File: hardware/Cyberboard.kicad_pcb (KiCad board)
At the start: 4 copper layers, 51 x 21 mm, 68 parts, among them J1 Conn_01x20, J2 Conn_01x20, SW1 SW_Push, SW2 SW_Push, U1 SZYY0402Y_C434450, U10 XL-1005UBC_C22355736, U2 TPD2EUSB30, U3 NX2012SA-32.768KHZ-STD-MUB-2, U4 STM32WB55RGVx, U5 BQ24072RGT, U6 TPS631000DRLR, U7 ICM-42688-PC, U8 BMP580, U9 DFE252012P-1R0M=P2, X1 NX2016SA-32MHZ-STD-CZS-5

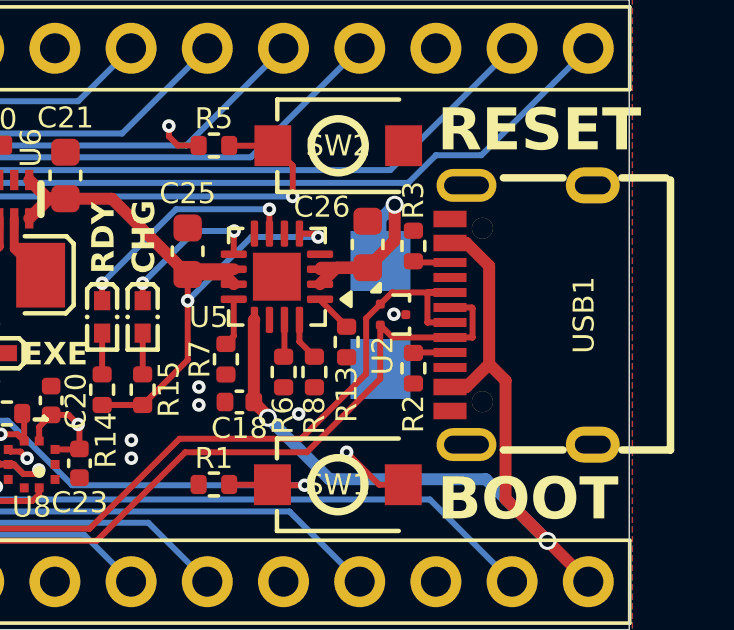
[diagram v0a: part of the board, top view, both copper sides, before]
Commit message: rounded corners and new renders and flyer
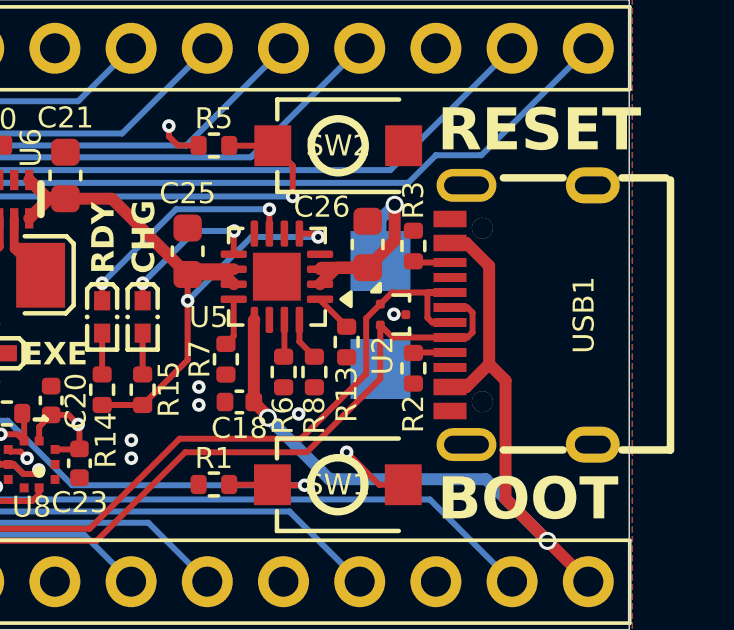
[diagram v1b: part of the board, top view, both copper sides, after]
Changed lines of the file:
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@@
+	)
+	(segment
+		(start 165.77 77.25)
+		(end 165.02 77.25)
+		(width 0.2)
+		(layer "F.Cu")
+		(net 27)
 	)
 	(segment
@@
 	)
 	(segment
+		(start 165.019 77.251)
+		(end 165.019 78.094)
+		(width 0.2)
+		(layer "F.Cu")
+		(net 27)
+	)
+	(segment
+		(start 165.019 78.094)
+		(end 165.175 78.25)
+		(width 0.2)
+		(layer "F.Cu")
+		(net 27)
+	)
+	(segment
 		(start 156.756802 82.125)
 		(end 160.806802 82.125)
@@
 	)
 	(segment
-		(start 165.77 77.25)
-		(end 165.02 77.25)
-		(width 0.2)
-		(layer "F.Cu")
-		(net 27)
-	)
-	(segment
-		(start 165.019 78.249)
-		(end 165.02 78.25)
+		(start 165.175 78.25)
+		(end 165.77 78.25)
 		(width 0.2)
 		(layer "F.Cu")
@@
 	)
 	(segment
-		(start 165.02 78.25)
-		(end 165.77 78.25)
-		(width 0.2)
-		(layer "F.Cu")
-		(net 27)
-	)
-	(segment
-		(start 165.019 77.251)
-		(end 165.019 78.249)
-		(width 0.2)
-		(layer "F.Cu")
-		(net 27)
-	)
-	(segment
 		(start 150.375 84.95)
 		(end 150.55 85.125)
@@
 	)
 	(segment
-		(start 166.521 78.749)
-		(end 166.52 78.75)
-		(width 0.2)
-		(layer "F.Cu")
-		(net 28)
-	)
-	(segment
-		(start 165.77 77.75)
-		(end 166.5 77.75)
+		(start 166.521 77.921)
+		(end 166.521 78.579)
+		(width 0.2)
+		(layer "F.Cu")
+		(net 28)
+	)
+	(segment
+		(start 166.35 77.75)
+		(end 166.521 77.921)
 		(width 0.2)
 		(layer "F.Cu")
@@
 	)
 	(segment
+		(start 165.77 77.75)
+		(end 166.35 77.75)
+		(width 0.2)
+		(layer "F.Cu")
+		(net 28)
+	)
+	(segment
 		(start 165.77 78.75)
 		(end 163.86 78.75)
@@
 	)
 	(segment
+		(start 166.35 78.75)
+		(end 165.77 78.75)
+		(width 0.2)
+		(layer "F.Cu")
+		(net 28)
+	)
+	(segment
 		(start 160.993198 82.575)
 		(end 156.943198 82.575)
@@
 	)
 	(segment
-		(start 166.521 77.771)
-		(end 166.521 78.749)
-		(width 0.2)
-		(layer "F.Cu")
-		(net 28)
-	)
-	(segment
 		(start 140.599517 85.525)
 		(end 138.036136 82.961619)
@@
 	)
 	(segment
-		(start 166.52 78.75)
-		(end 165.77 78.75)
-		(width 0.2)
-		(layer "F.Cu")
-		(net 28)
-	)
-	(segment
-		(start 166.5 77.75)
-		(end 166.521 77.771)
-		(width 0.2)
-		(layer "F.Cu")
-		(net 28)
-	)
-	(segment
 		(start 163.4475 78.3375)
 		(end 163.4475 80.120698)
@@
 		(width 0.2)
 		(layer "F.Cu")
+		(net 28)
+	)
+	(segment
+		(start 166.521 78.579)
+		(end 166.35 78.75)
+		(width 0.2)
+		(layer "F.Cu")
